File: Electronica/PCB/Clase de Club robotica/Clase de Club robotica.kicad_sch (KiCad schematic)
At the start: 18 parts, among them J1 Ultrasonico 1, J3 Ultrasonico 2, J4 Ultrasonico 3, J5 Ultrasonico 4, SW1 SW_SPST, SW2 SW_Push, U1 CNY70, U2 CNY70

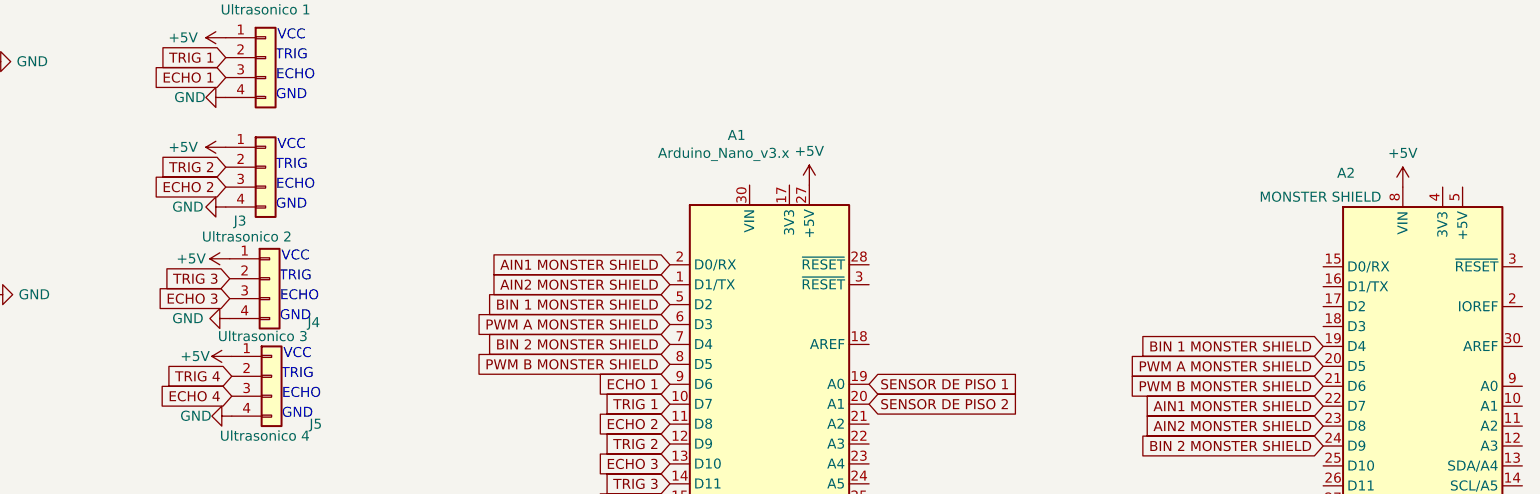
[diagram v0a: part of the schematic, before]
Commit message: Inicio de diseño del pcb
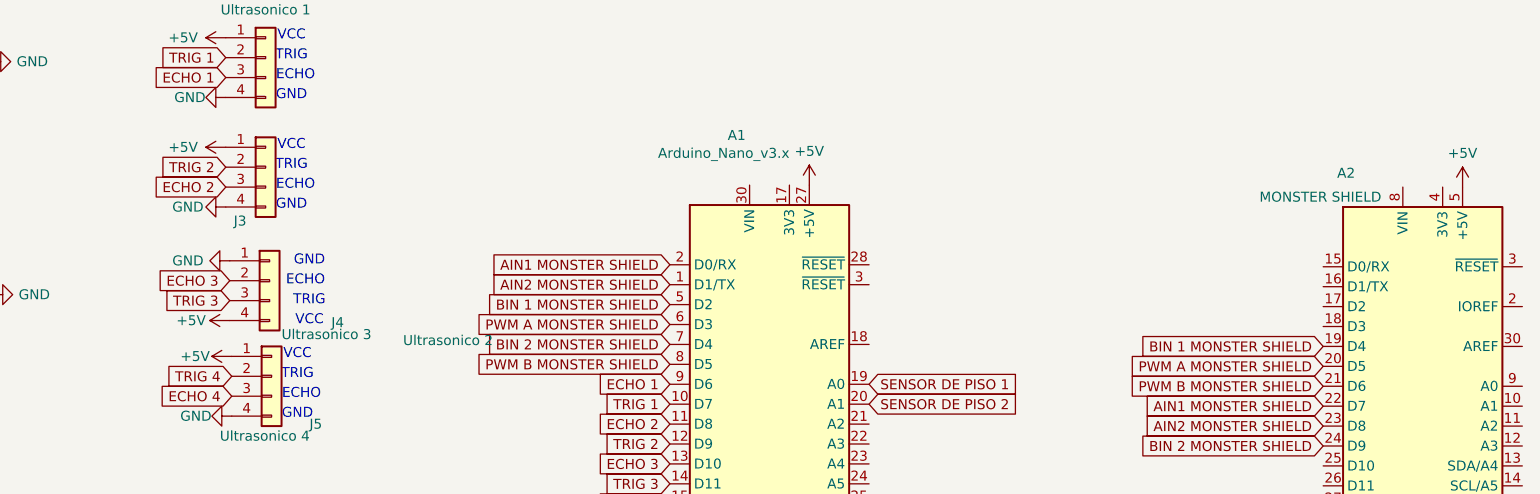
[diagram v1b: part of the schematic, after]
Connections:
- net +5V: now also A2.5 (+5V), J4.4 (Pin_4); no longer A2.8 (VIN), J4.1 (Pin_1)
- net ECHO 3: now also J4.2 (Pin_2); no longer J4.3 (Pin_3)
- net GND: now also J4.1 (Pin_1); no longer J4.4 (Pin_4)
- net TRIG 3: now also J4.3 (Pin_3); no longer J4.2 (Pin_2)

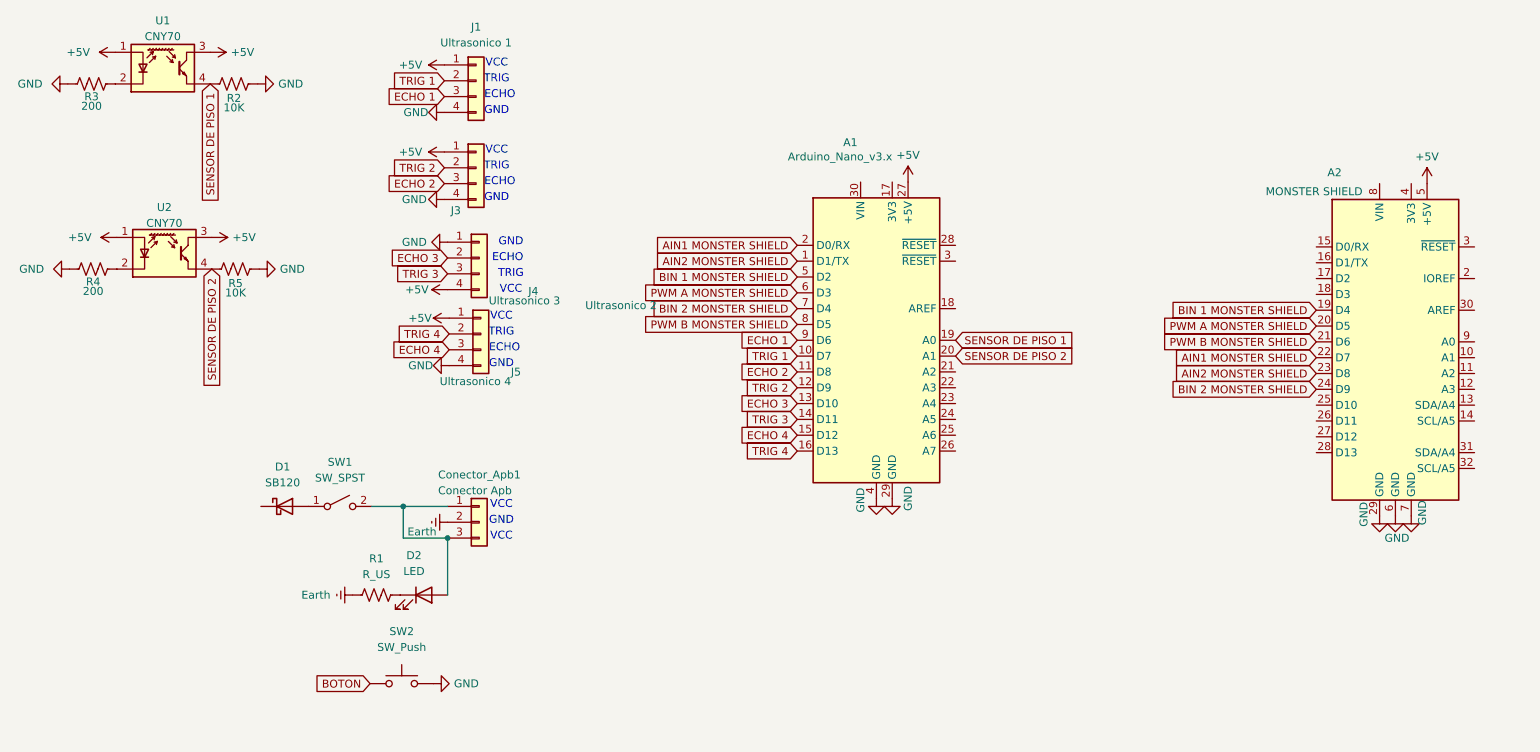
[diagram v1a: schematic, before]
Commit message: Esquematico correjido por prieto solo falta el step up y step down
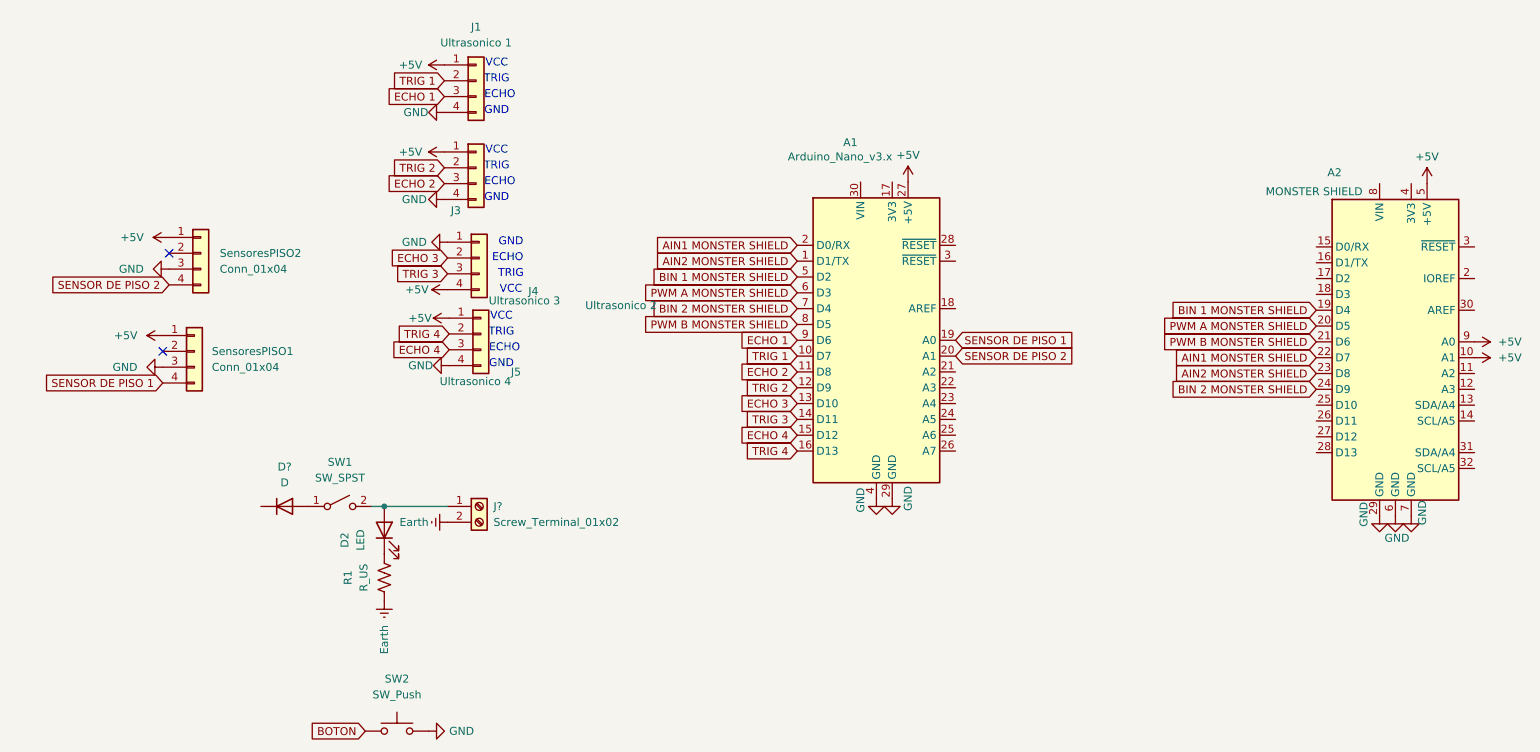
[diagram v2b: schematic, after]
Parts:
- removed Conector_Apb1: Conector Apb, Connector_PinHeader_2.54mm:PinHeader_1x03_P2.54mm_Vertical, symbol Connector_Generic:Conn_01x03
- removed D1: SB120, Diode_THT:D_DO-41_SOD81_P10.16mm_Horizontal, symbol Diode:SB120
- removed R2, R5: 10K, Resistor_THT:R_Axial_DIN0207_L6.3mm_D2.5mm_P10.16mm_Horizontal, symbol Device:R_US
- removed R3, R4: 200, Resistor_THT:R_Axial_DIN0207_L6.3mm_D2.5mm_P10.16mm_Horizontal, symbol Device:R_US
- removed U1, U2: CNY70, Connector_PinHeader_2.54mm:PinHeader_1x04_P2.54mm_Vertical, symbol Sensor_Proximity:CNY70
- added D?: D, symbol Device:D
- added J?: Screw_Terminal_01x02, symbol Connector:Screw_Terminal_01x02
- added SensoresPISO1, SensoresPISO2: Conn_01x04, Connector_PinSocket_2.54mm:PinSocket_1x04_P2.54mm_Vertical, symbol Connector_Generic:Conn_01x04
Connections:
- net +5V: now also A2.10 (A1), A2.9 (A0), SensoresPISO1.1 (Pin_1), SensoresPISO2.1 (Pin_1)
- net Earth: now also J?.2 (Pin_2)
- net GND: now also SensoresPISO1.3 (Pin_3), SensoresPISO2.3 (Pin_3)
- net SENSOR DE PISO 1: now also SensoresPISO1.4 (Pin_4)
- net SENSOR DE PISO 2: now also SensoresPISO2.4 (Pin_4)
- net at D2.2 (A), SW1.2 (B): now also J?.1 (Pin_1)
- net at SW1.1 (A): now also D?.2 (A)
- no-connect marks 0 -> 2
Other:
- moved on the sheet: D2, R1, SW2
